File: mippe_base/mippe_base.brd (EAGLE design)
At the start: 160 x 100 mm, 17 parts, among them IC1 ATMEGA168PROUND, SW1 BTN-PTS810

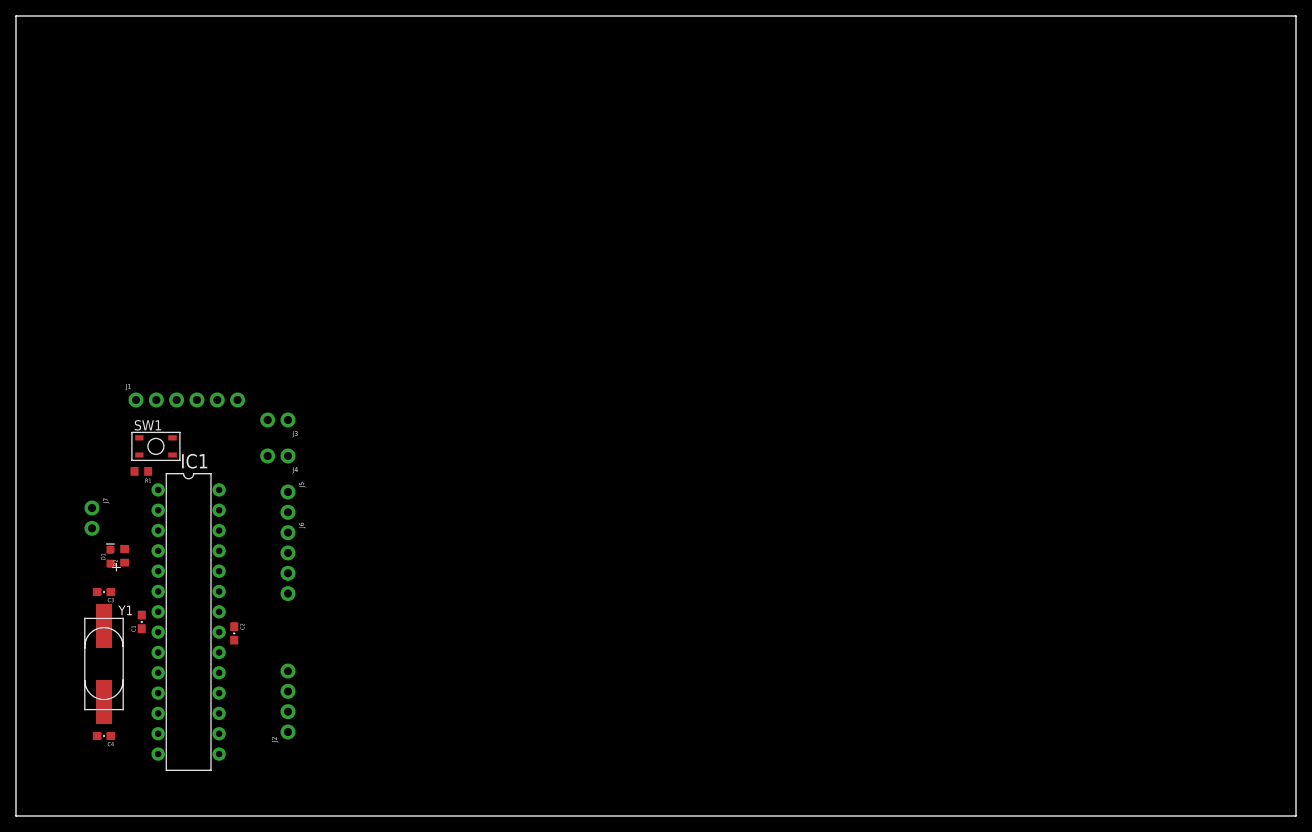
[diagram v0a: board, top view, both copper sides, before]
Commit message: Finish burnin and mippe controller
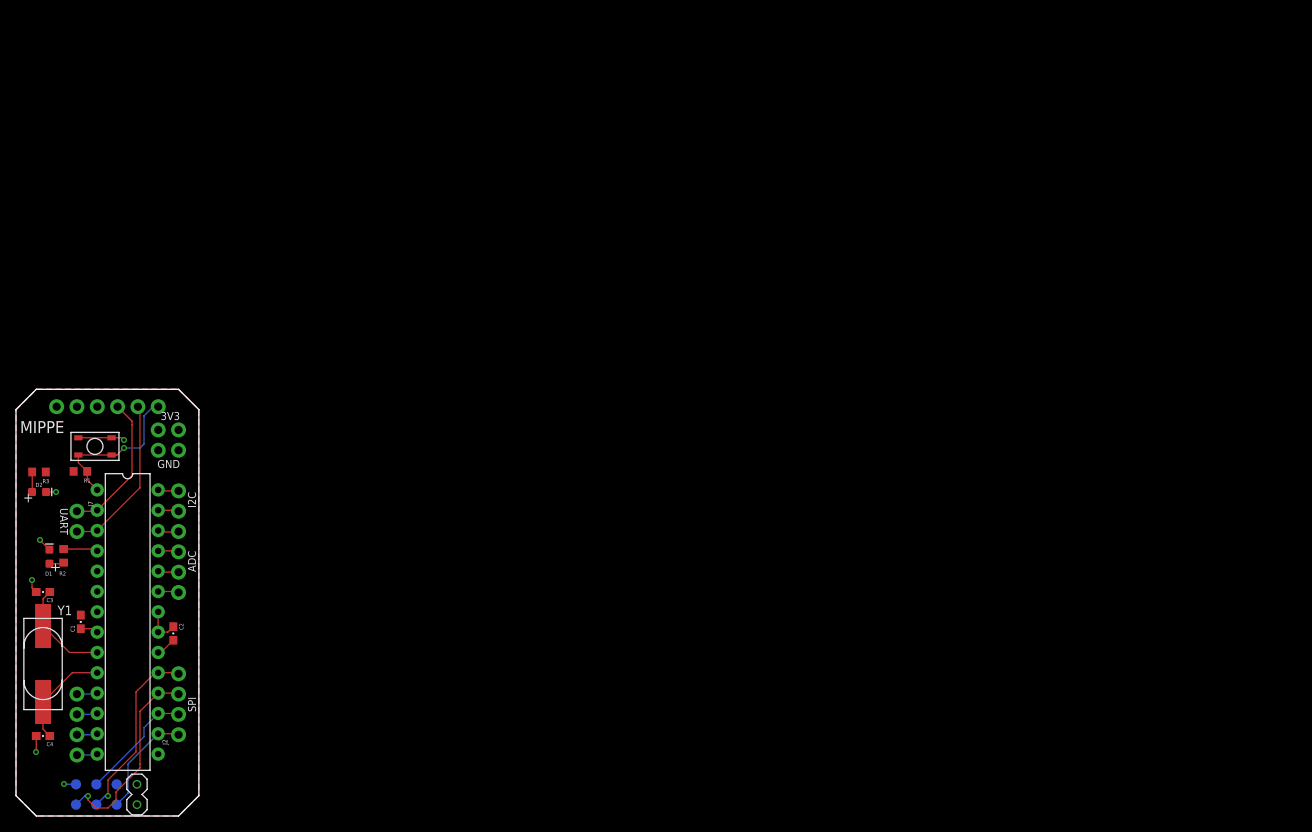
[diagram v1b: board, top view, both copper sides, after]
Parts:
- added D2: RED, scono:LED-0603
- added J8: (no value), scono:1X04_NO_SILK
- added J9: BURNIN, scono:BURNIN
- added R3: 330R, scono:R0603
- R2: value (none) -> 330R
- Y1: value (none) -> 16MHz
- moved J3 13.7 mm to (20.3, 48.3)
- moved J4 13.7 mm to (20.3, 45.7)
- moved J2 13.7 mm to (20.3, 10.2)
- moved J5 13.7 mm to (20.3, 40.6)
- moved J6 13.7 mm to (20.3, 35.6)
- moved J1 9.96 mm to (5.08, 51.2)
- moved C1 7.62 mm to (8.10, 24.3)
- moved C2 7.62 mm to (19.7, 22.8)
- moved D1 7.62 mm to (4.18, 32.4)
- moved C3 7.62 mm to (3.38, 28.0)
- moved C4 7.62 mm to (3.38, 10.0)
- moved R2 7.62 mm to (5.95, 32.5)
- moved Y1 7.62 mm to (3.38, 19.0)
- moved R1 7.62 mm to (8.05, 43.1)
- moved SW1 7.62 mm to (9.87, 46.2)
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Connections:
- removed net DTR: J1.6
- new net N$2: D2.A, R3.2
- net 3.3V: now also J9.3.3V, R3.1
- net GND: now also D2.C, J9.GND
- net GPIO3: now also J8.4
- net GPIO4: now also J8.3
- net GPIO5: now also J8.2
- net GPIO6: now also J8.1
- net MISO: now also J9.MISO
- net MOSI: now also J9.MOSI
- net RST: now also J1.6
- net SCK: now also J9.SCK
- net SS: now also J9.SS
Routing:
- net MISO: track 0.00 -> 24.9 mm, vias 0 -> 1
- net SCK: track 0.00 -> 22.7 mm, vias 0 -> 1
- net TX: track 0.00 -> 20.8 mm
- net RST: track 0.00 -> 19.9 mm, vias 0 -> 1
- net GND: track 0.00 -> 19.4 mm, vias 0 -> 5
- net RX: track 0.00 -> 18.1 mm
- net MOSI: track 0.00 -> 14.7 mm
- net SS: track 0.00 -> 13.6 mm
- net N$4: track 0.00 -> 12.9 mm
- net N$3: track 0.00 -> 12.7 mm
- net GPIO0: track 0.00 -> 4.30 mm
- net 3.3V: track 0.00 -> 4.04 mm, vias 0 -> 1
- net ADC3: track 0.00 -> 2.65 mm
- net ADC1: track 0.00 -> 2.60 mm
- net SDA: track 0.00 -> 2.60 mm
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- added copper zone on layer 1, net 3.3V
- added copper zone on layer 16, net GND
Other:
- board size 160 x 100 mm -> 22.9 x 53.3 mm
- board text added: "3V3"
- board text added: "ADC"
- board text added: "Arduino Bootloader Burnin"
- board text added: "Arduino Uno Redesign Fa19"
- board text added: "Arias Research Group Seiya Ono"
- board text added: "GND"
- board text added: "I2C"
- board text added: "MIPPE"
- board text added: "SPI"
- board text added: "UART"
- board text added: "USB to TTL Interface"
